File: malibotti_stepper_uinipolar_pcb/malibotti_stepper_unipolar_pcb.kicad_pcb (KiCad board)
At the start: 2 copper layers, 70 x 68 mm, 35 parts, among them J1 Stepper 1, J2 Stepper 2, J3 Servo, J4 I2C, J5 USB_C_Receptacle_USB2.0_16P, J6 Serial, SW1 RST, SW2 MicroSwitchLeft, SW3 MicroSwitchRight, SW8 BTN, U1 TBD62783A, U3 AMS1117, U5 ESP32-S3-MINI-1

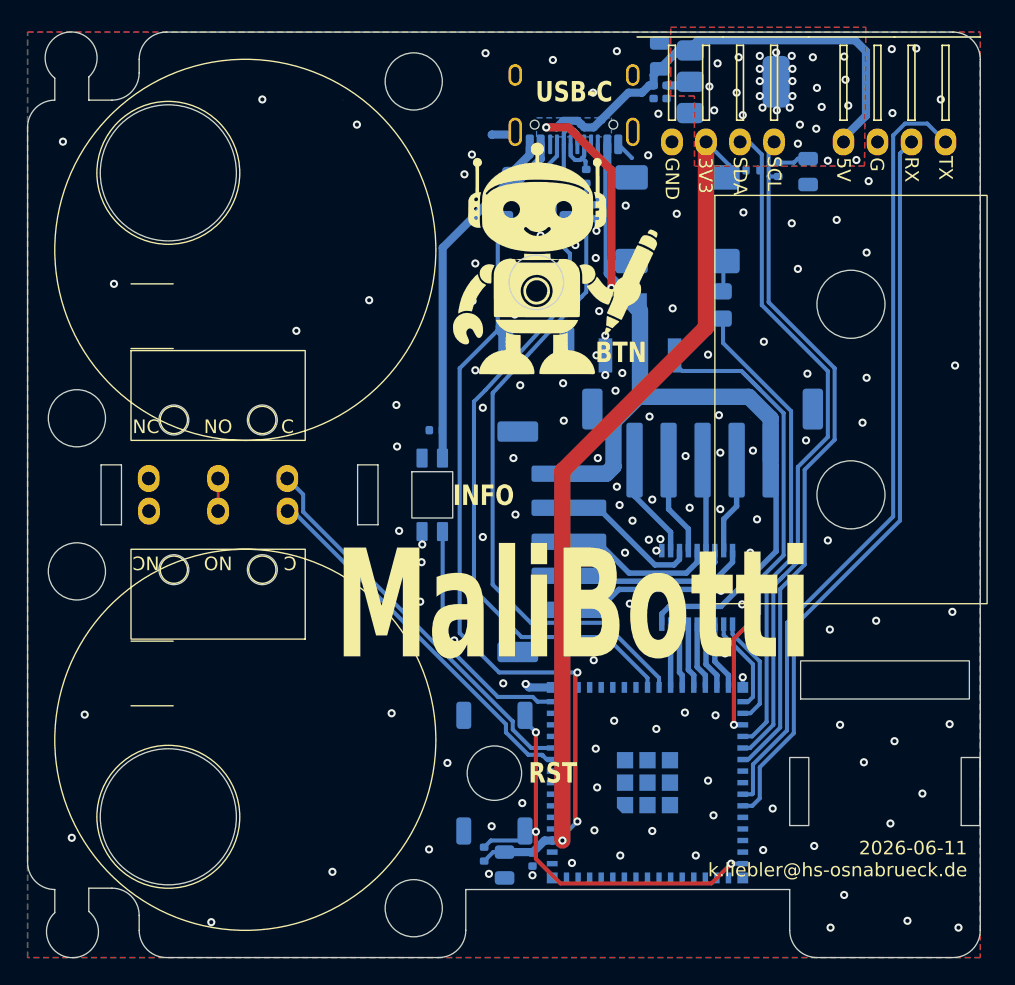
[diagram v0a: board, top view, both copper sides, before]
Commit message: Varions
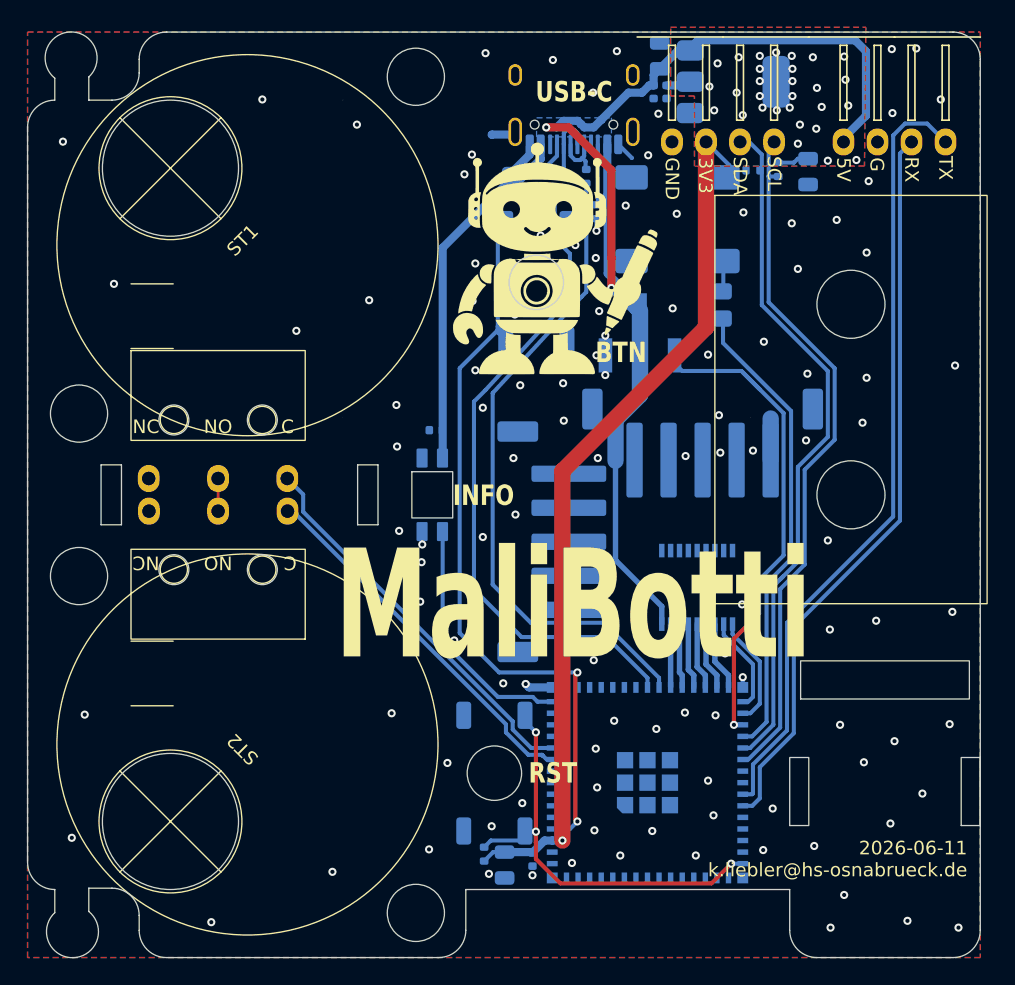
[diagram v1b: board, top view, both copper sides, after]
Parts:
- moved ST1 8.14 mm to (60.5, 76.0)
- moved ST2 8.14 mm to (60.5, 124.0)
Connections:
- J1 pad 1: Net-(J1-Pin_1) -> GND
- J1 pad 5: +5V -> Net-(J1-Pin_5)
- J2 pad 1: Net-(J2-Pin_1) -> GND
- J2 pad 5: +5V -> Net-(J2-Pin_5)
- U1 pad 11: Net-(J1-Pin_1) -> Net-(J1-Pin_5)
- U1 pad 12: Net-(J2-Pin_4) -> Net-(J2-Pin_2)
- U1 pad 13: Net-(J1-Pin_2) -> Net-(J1-Pin_4)
- U1 pad 16: Net-(J2-Pin_2) -> Net-(J2-Pin_4)
- U1 pad 17: Net-(J1-Pin_4) -> Net-(J1-Pin_2)
- U1 pad 18: Net-(J2-Pin_1) -> Net-(J2-Pin_5)
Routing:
- net +5V: track 139.3 -> 117.4 mm
- net Net-(J2-Pin_1): track 14.3 -> 0.00 mm
- net Net-(J2-Pin_2): track 12.3 -> 0.00 mm
- net Net-(J2-Pin_3): track 11.6 -> 0.00 mm
- net Net-(J2-Pin_4): track 10.7 -> 0.00 mm
- net Net-(J1-Pin_1): track 7.75 -> 0.00 mm
- net Net-(J1-Pin_2): track 7.25 -> 0.00 mm
- net Net-(J1-Pin_4): track 7.04 -> 0.00 mm
- net Net-(J1-Pin_3): track 6.75 -> 0.00 mm
- net Net-(J1-Pin_5): track 0.00 -> 3.06 mm
- net GND: vias 136 -> 119
